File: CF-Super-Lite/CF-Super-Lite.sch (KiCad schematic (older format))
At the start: 11 parts, among them J1 Bus_ISA_8bit, J2 ATA_CONNECTOR, SW1 DIP Switch x3 or x4, U1 BIOS FLASH, U2 74HCT245, U3 GAL16V8

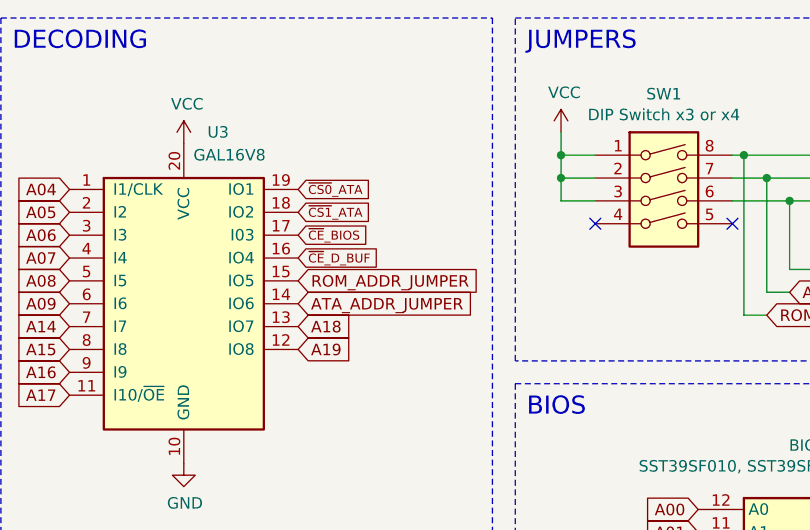
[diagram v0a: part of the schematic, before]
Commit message: More premature layout work.
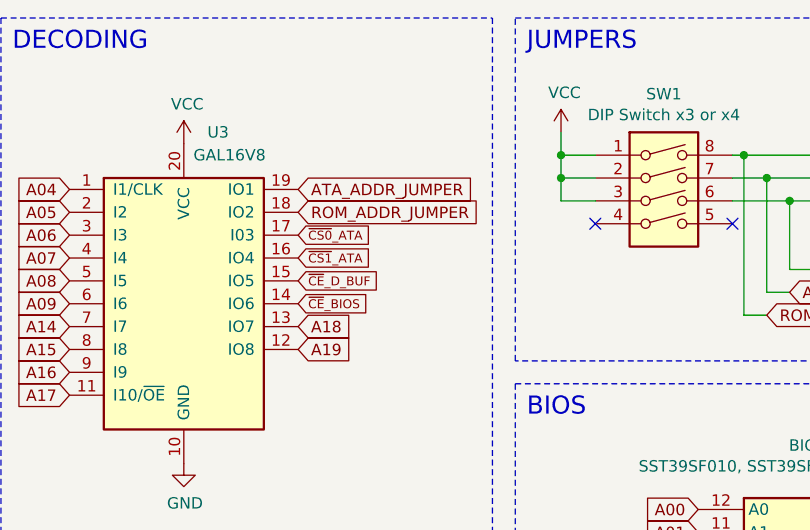
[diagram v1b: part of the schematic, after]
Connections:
- net ATA_ADDR_JUMPER: now also U3.19 (IO1); no longer U3.14 (IO6)
- net ROM_ADDR_JUMPER: now also U3.18 (IO2); no longer U3.15 (IO5)
- net ~CE~_BIOS: now also U3.14 (IO6); no longer U3.17 (I03)
- net ~CE~_D_BUF: now also U3.15 (IO5); no longer U3.16 (IO4)
- net ~CS0~_ATA: now also U3.17 (I03); no longer U3.19 (IO1)
- net ~CS1~_ATA: now also U3.16 (IO4); no longer U3.18 (IO2)
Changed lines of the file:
@@
 Text GLabel 7600 3500 2    50   Input ~ 0
 D7_BUF
-Text GLabel 4650 1400 2    39   Input ~ 0
+Text GLabel 4650 1600 2    39   Input ~ 0
 ~CS0~_ATA
-Text GLabel 4650 1500 2    39   Input ~ 0
+Text GLabel 4650 1700 2    39   Input ~ 0
 ~CS1~_ATA
-Text GLabel 4650 1600 2    39   Input ~ 0
+Text GLabel 4650 1900 2    39   Input ~ 0
 ~CE~_BIOS
-Text GLabel 4650 1700 2    39   Input ~ 0
+Text GLabel 4650 1800 2    39   Input ~ 0
 ~CE~_D_BUF
 Text GLabel 2700 3500 2    50   Input ~ 0
@@
 Text GLabel 3650 2000 0    50   Input ~ 0
 A14
-Text GLabel 4650 1800 2    50   Input ~ 0
+Text GLabel 4650 1500 2    50   Input ~ 0
 ROM_ADDR_JUMPER
-Text GLabel 4650 1900 2    50   Input ~ 0
+Text GLabel 4650 1400 2    50   Input ~ 0
 ATA_ADDR_JUMPER
 Text GLabel 6400 4300 0    50   Input ~ 0
